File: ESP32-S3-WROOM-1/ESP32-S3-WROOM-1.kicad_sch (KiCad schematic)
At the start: 23 parts, among them J1 ESP32-S3-DEVKITC-1-J1, J2 ESP32-S3-DEVKITC-1-J2, J3 UART, P1 USB2.0_C_12pin, SW1 BOOT, SW2 RESET, U1 ESP32-S3-WROOM-1, U2 AMS1117-3.3

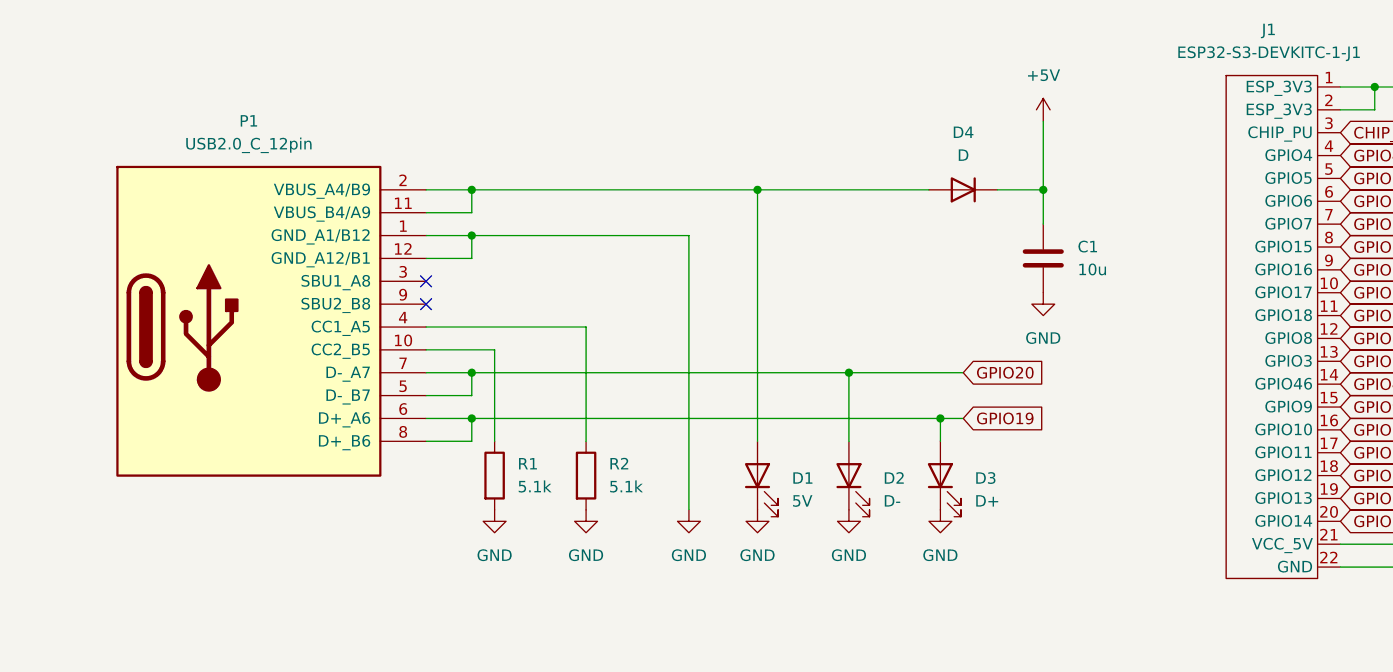
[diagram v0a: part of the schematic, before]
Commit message: fix
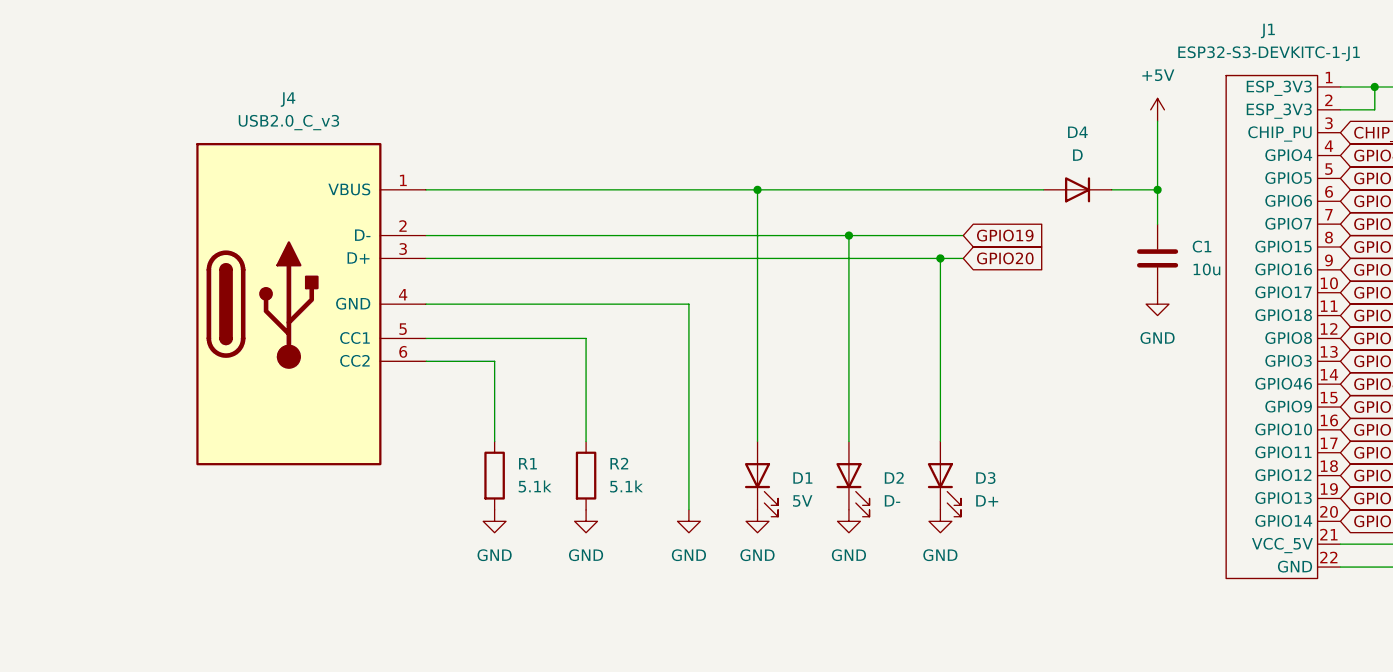
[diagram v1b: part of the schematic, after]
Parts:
- removed P1: USB2.0_C_12pin, esp32-dev-boards:USB-C-12-Pin-MidMount, symbol $74th:USB2.0_C_12pin
- added J4: USB2.0_C_v3, $74th:USB-C-12-Pin-MidMount-ali-v4, symbol $74th:USB2.0_C_v3
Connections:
- net GND: now also J4.4 (GND)
- net GPIO19: now also D2.2 (A), J4.2 (D-); no longer D3.2 (A)
- net GPIO20: now also D3.2 (A), J4.3 (D+); no longer D2.2 (A)
- net at D1.2 (A), D4.2 (A): now also J4.1 (VBUS)
- net at R1.1: now also J4.6 (CC2)
- net at R2.1: now also J4.5 (CC1)
- no-connect marks 2 -> 0
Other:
- moved on the sheet: C1, D4
